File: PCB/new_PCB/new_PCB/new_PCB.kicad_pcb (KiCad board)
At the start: 2 copper layers, 127 x 102.2 mm, 18 parts, among them J1 XT60PW-F, J2 XT60PW-F, J3 MOLEX-Connector, J4 MOLEX-Connector, J5 MOLEX-Connector, J6 MOLEX-Connector, J7 MOLEX-Connector, J8 MOLEX-Connector, U1 ESP32-S3-DEVKITC-1-N16R8V

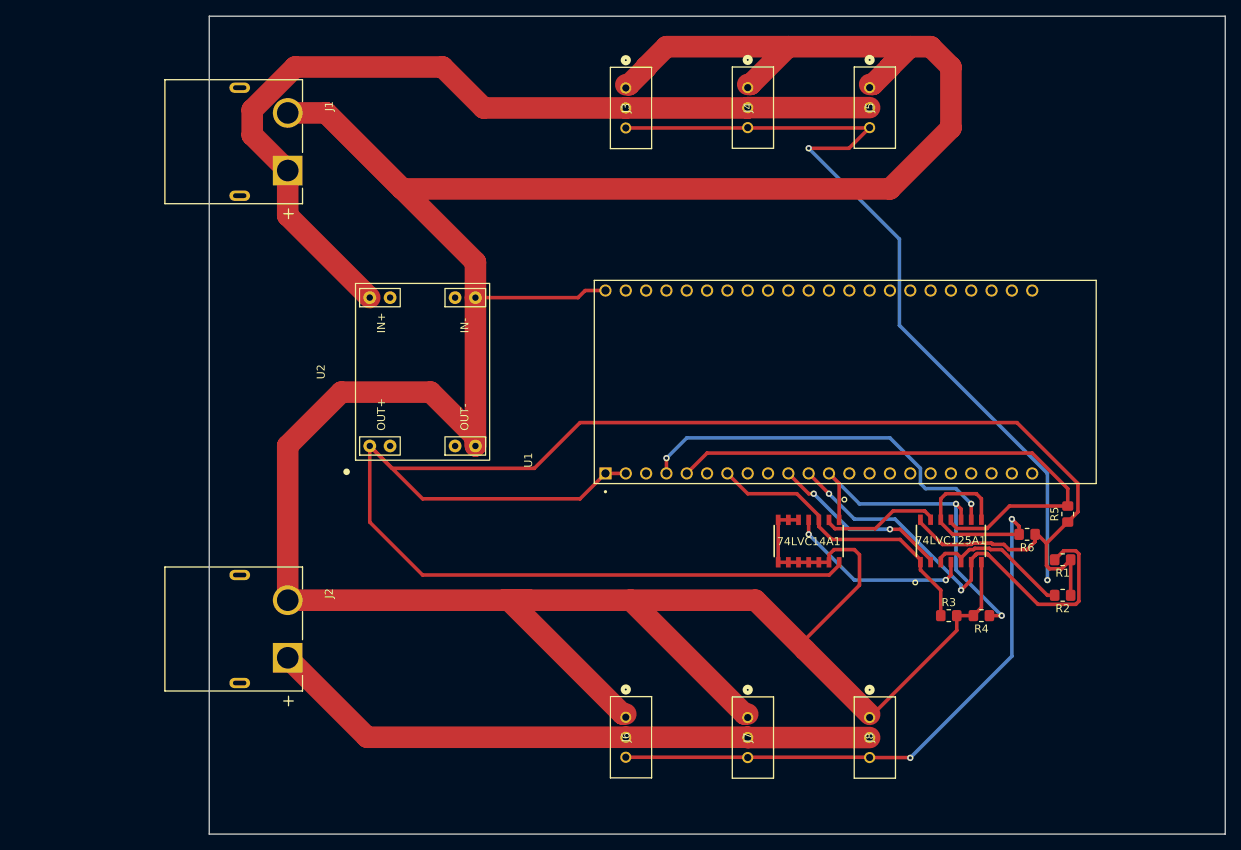
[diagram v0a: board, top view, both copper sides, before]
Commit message: Add changes to new pcb
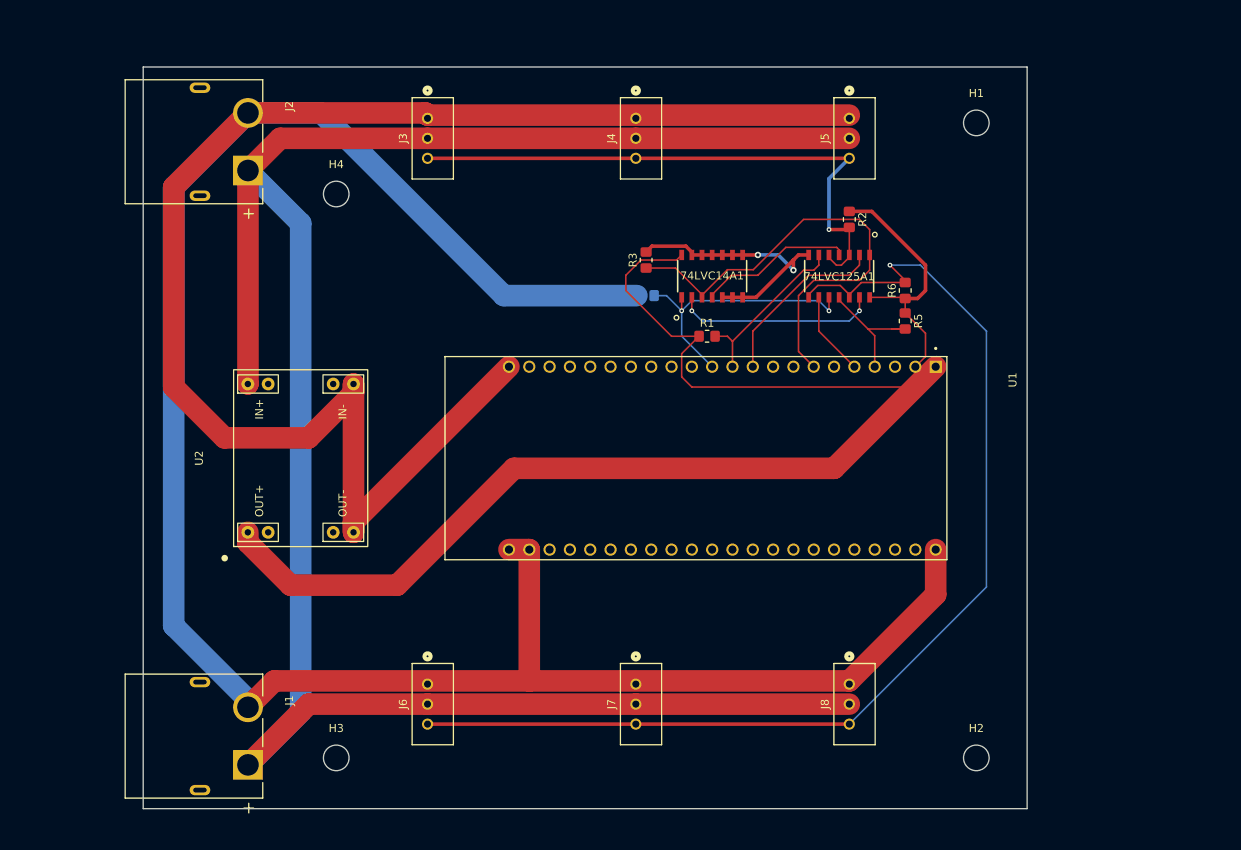
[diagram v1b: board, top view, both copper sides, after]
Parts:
- added H1: MountingHole, MountingHole:MountingHole_3.2mm_M3_ISO14580, F.Cu at (137.8, 29.8)
- added H2: MountingHole, MountingHole:MountingHole_3.2mm_M3_ISO14580, F.Cu at (137.8, 109.2)
- added H3: MountingHole, MountingHole:MountingHole_3.2mm_M3_ISO14580, F.Cu at (57.8, 109.2)
- added H4: MountingHole, MountingHole:MountingHole_3.2mm_M3_ISO14580, F.Cu at (57.8, 38.7)
- R4: moved to B.Cu
- moved J1 74.5 mm to (46.8, 106.5)
- moved J2 61.1 mm to (46.8, 32.2)
- moved R3 58.4 mm to (96.5, 47.0), turned to 90 degrees
- moved R4 57.9 mm to (96.5, 51.4)
- moved R2 54.0 mm to (121.9, 41.9), turned to -90 degrees
- moved R1 52.5 mm to (104.1, 56.5), turned to 0 degrees
- moved 74LVC125A1 38.9 mm to (124.5, 46.4), turned to -90 degrees
- moved R6 34.1 mm to (128.9, 50.8), turned to 90 degrees
- moved 74LVC14A1 34.1 mm to (101.0, 51.7), turned to 90 degrees
- moved R5 31.5 mm to (128.9, 54.6), turned to -90 degrees
- moved J6 25.1 mm to (69.2, 100.0)
- moved J3 25.1 mm to (69.2, 29.3)
- moved U1 21.0 mm to (102.7, 71.8), turned to -90 degrees
- moved U2 18.7 mm to (53.3, 71.8)
- moved J7 14.6 mm to (95.2, 100.0)
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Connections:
- U1 pad J1_22: (no net) -> GND
- U1 pad J1_4: /TX2 -> /RX2
- U1 pad J1_5: /RX2 -> /TX2
- U1 pad J3_21: (no net) -> GND
- U1 pad J3_22: (no net) -> GND
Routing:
- net VBUS: track 188.0 -> 261.6 mm
- net /RX2: track 69.1 -> 16.8 mm
- net /SERVO_DATA1: track 124.2 -> 72.7 mm, vias 2 -> 1
- net /SERVO_DATA2: track 94.6 -> 141.7 mm, vias 2 -> 1
- net +3.3V: track 242.5 -> 195.7 mm
- net /TX2: track 47.6 -> 10.5 mm, vias 2 -> 0
- net /RX1: track 56.1 -> 21.6 mm, vias 2 -> 0
- net GND: track 454.5 -> 480.1 mm, vias 0 -> 2
- net /TXEN1: track 37.4 -> 59.4 mm
- net /RXEN2: track 14.9 -> 25.4 mm, vias 0 -> 2
- net /TXEN2: track 43.9 -> 35.6 mm
- net /RXEN1: track 23.8 -> 19.4 mm, vias 2 -> 0
- net /TX1: vias 2 -> 0
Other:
- board size 127 x 102.2 mm -> 110.5 x 92.7 mm

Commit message: Final PCB version
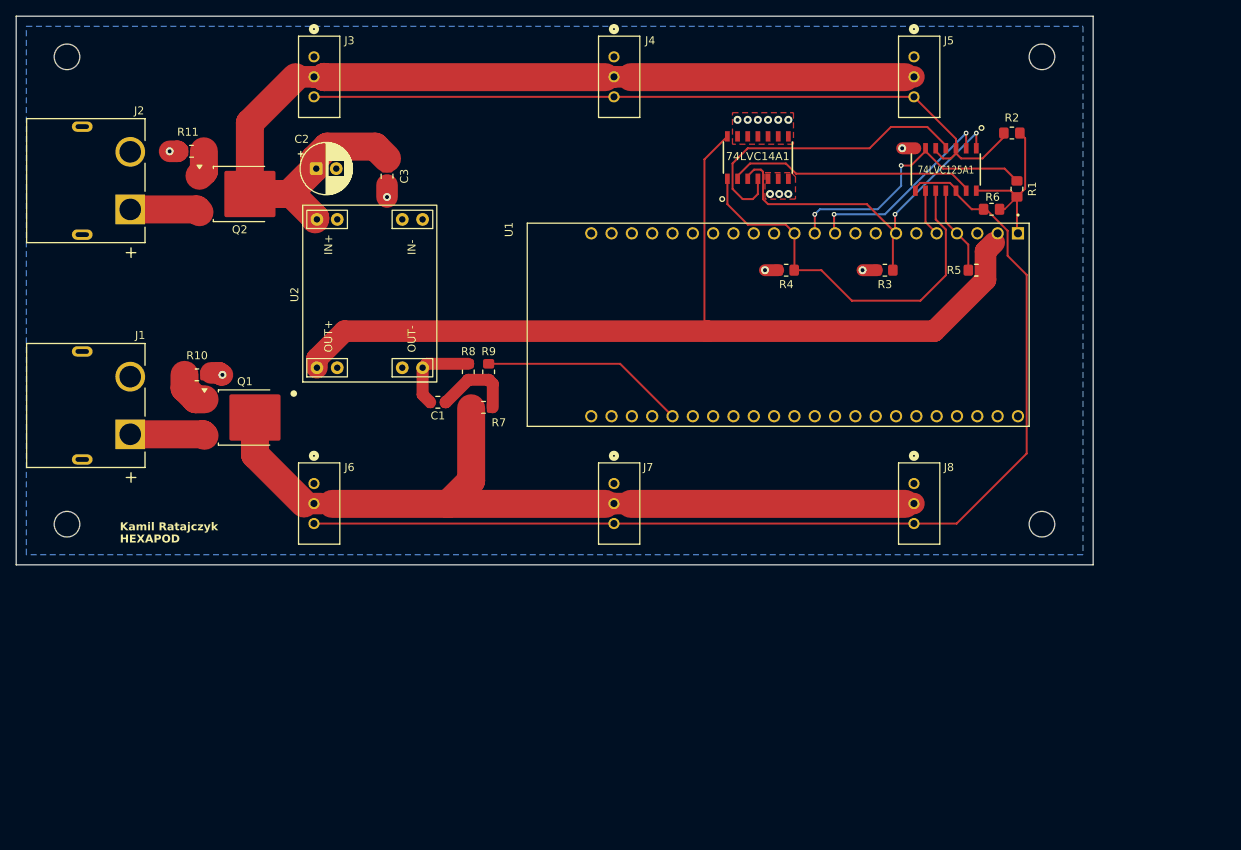
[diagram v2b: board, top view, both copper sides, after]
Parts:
- added C1: 100nF, Capacitor_SMD:C_0805_2012Metric, F.Cu at (70.5, 64.8)
- added C2: 100uF, Capacitor_THT:CP_Radial_D6.3mm_P2.50mm, F.Cu at (55.3, 35.6)
- added C3: 100nF, Capacitor_SMD:C_0805_2012Metric, F.Cu at (64.1, 36.5)
- added Q1: Q_PMOS, Package_TO_SOT_SMD:TO-252-2, F.Cu at (46.4, 66.7)
- added Q2: Q_PMOS, Package_TO_SOT_SMD:TO-252-2, F.Cu at (45.7, 38.7)
- added R10: 10k, Resistor_SMD:R_0805_2012Metric_Pad1.20x1.40mm_HandSolder, F.Cu at (40.4, 61.3)
- added R11: 10k, Resistor_SMD:R_0805_2012Metric_Pad1.20x1.40mm_HandSolder, F.Cu at (39.7, 33.4)
- added R7: 100k, Resistor_SMD:R_0805_2012Metric_Pad1.20x1.40mm_HandSolder, F.Cu at (76.2, 65.4)
- added R8: 22k, Resistor_SMD:R_0805_2012Metric_Pad1.20x1.40mm_HandSolder, F.Cu at (74.3, 61.0)
- added R9: 1k, Resistor_SMD:R_0805_2012Metric_Pad1.20x1.40mm_HandSolder, F.Cu at (76.8, 61.0)
- R4: moved to F.Cu
- moved H2 143.5 mm to (24.1, 21.6)
- moved H3 92.9 mm to (146.0, 80.0)
- moved H4 53.3 mm to (24.1, 80.0)
- moved J1 43.9 mm to (32.0, 65.2)
- moved R1 42.9 mm to (142.9, 38.1), turned to 90 degrees
- moved R3 29.9 mm to (126.4, 48.3), turned to 180 degrees
- moved J6 28.8 mm to (55.0, 74.9)
- moved J8 26.3 mm to (130.0, 74.9)
- moved J7 25.2 mm to (92.5, 74.9)
- moved R2 23.0 mm to (142.2, 31.1), turned to 180 degrees
- moved U2 22.3 mm to (62.0, 51.2)
- moved U1 19.6 mm to (113.0, 55.1)
- moved 74LVC125A1 18.9 mm to (137.8, 33.0)
- moved R4 17.8 mm to (114.0, 48.3)
- moved J3 16.1 mm to (55.0, 21.6)
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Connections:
- J1 pad 1: VBUS -> VBAT
- J2 pad 1: VBUS -> VBAT
- J3 pad 2: VBUS -> VBUS_2
- J4 pad 2: VBUS -> VBUS_2
- J5 pad 2: VBUS -> VBUS_2
- J6 pad 2: VBUS -> VBUS_1
- J7 pad 2: VBUS -> VBUS_1
- J8 pad 2: VBUS -> VBUS_1
- U1 pad J3_18: unconnected-(U1-GPIO21-PadJ3_18) -> /BAT_LVL
- U2 pad 8: VBUS -> VBUS_2
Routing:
- net GND: track 480.1 -> 19.8 mm, vias 2 -> 15
- net VBUS: track 261.6 -> 0.00 mm
- net VBUS_2: track 0.00 -> 119.6 mm
- net VBUS_1: track 0.00 -> 100.1 mm
- net +3.3V: track 195.7 -> 146.5 mm
- net /BAT_LVL: track 0.00 -> 25.7 mm
- net /SERVO_DATA1: track 72.7 -> 95.6 mm, vias 1 -> 0
- net /RXEN1: track 19.4 -> 38.9 mm
- net VBAT: track 0.00 -> 18.2 mm
- net /TXEN2: track 35.6 -> 50.6 mm, vias 2 -> 0
- net /RX1: track 21.6 -> 34.3 mm, vias 0 -> 2
- net /TXEN1: track 59.4 -> 48.0 mm, vias 0 -> 2
- net Net-(C1-Pad1): track 0.00 -> 10.2 mm
- net /RXEN2: track 25.4 -> 31.2 mm, vias 2 -> 0
- net /RX2: track 16.8 -> 11.1 mm
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- added copper zone on B.Cu, net GND
- added copper zone on F.Cu, net GND
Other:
- board size 110.5 x 92.7 mm -> 134.6 x 68.6 mm
- board text added: "HEXAPOD"
- board text added: "Kamil Ratajczyk"

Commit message: Final version of 2.0 PCB version
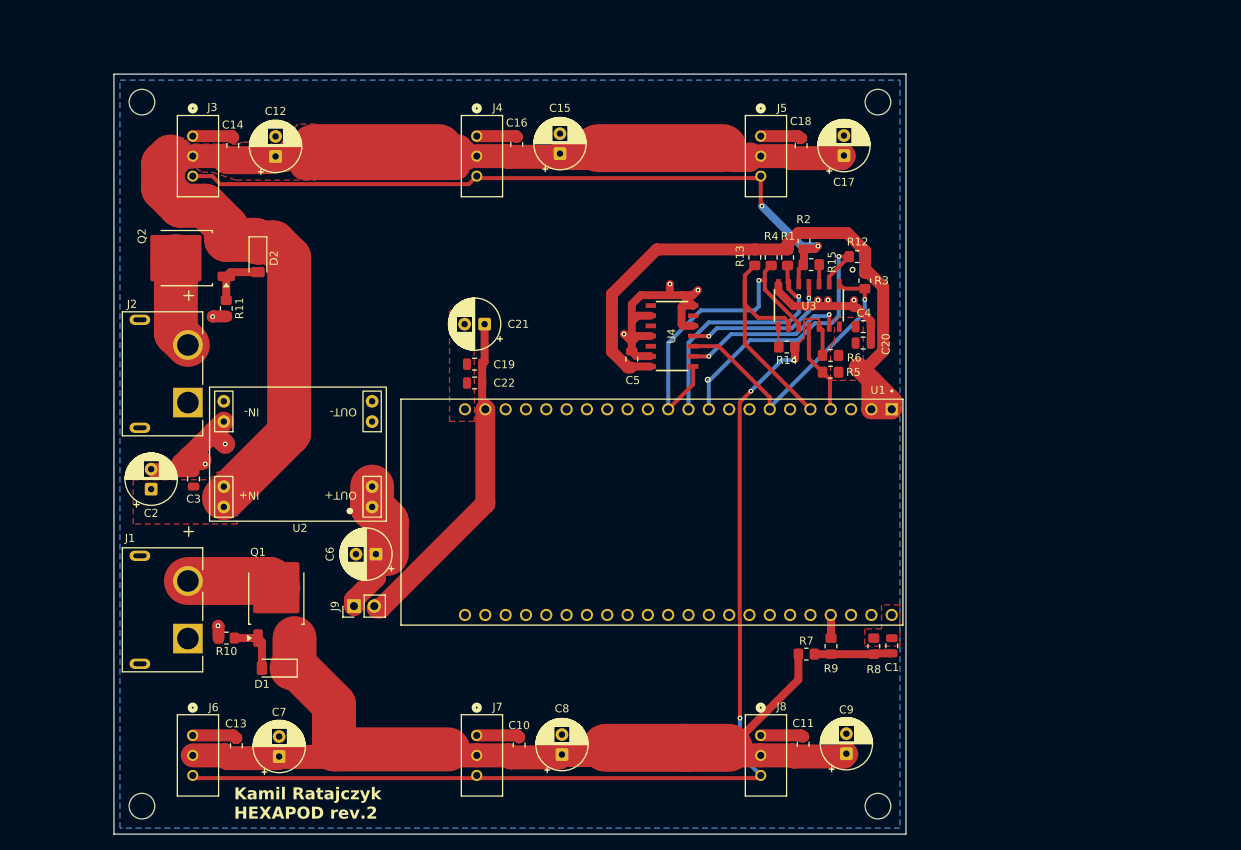
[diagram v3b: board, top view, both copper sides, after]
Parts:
- removed 74LVC125A1, 74LVC14A1: ~, Elements:SOT108-1
- added C10: 100nF, Capacitor_SMD:C_0805_2012Metric, F.Cu at (80.6, 107.6)
- added C11: 100nF, Capacitor_SMD:C_0805_2012Metric, F.Cu at (116.2, 107.5)
- added C12: 220uF, Capacitor_THT:CP_Radial_D6.3mm_P2.50mm, F.Cu at (50.2, 34.0)
- added C13: 100nF, Capacitor_SMD:C_0805_2012Metric, F.Cu at (45.3, 107.7)
- added C14: 100nF, Capacitor_SMD:C_0805_2012Metric, F.Cu at (44.9, 32.7)
- added C15: 220uF, Capacitor_THT:CP_Radial_D6.3mm_P2.50mm, F.Cu at (85.8, 33.7)
- added C16: 100nF, Capacitor_SMD:C_0805_2012Metric, F.Cu at (80.4, 32.5)
- added C17: 220uF, Capacitor_THT:CP_Radial_D6.3mm_P2.50mm, F.Cu at (121.2, 33.9)
- added C18: 100nF, Capacitor_SMD:C_0805_2012Metric, F.Cu at (115.9, 32.7)
- added C19: 10uF, Capacitor_SMD:C_0805_2012Metric, F.Cu at (75.1, 60.0)
- added C20: 10uF, Capacitor_SMD:C_0805_2012Metric, F.Cu at (123.7, 57.4)
- added C21: 220uF, Capacitor_THT:CP_Radial_D6.3mm_P2.50mm, F.Cu at (76.3, 55.0)
- added C22: 100nF, Capacitor_SMD:C_0805_2012Metric, F.Cu at (75.1, 62.4)
- added C4: 100nF, Capacitor_SMD:C_0805_2012Metric, F.Cu at (123.7, 55.3)
- added C5: 100nF, Capacitor_SMD:C_0805_2012Metric, F.Cu at (94.7, 59.4)
- added C6: 22uF, Capacitor_THT:CP_Radial_D6.3mm_P2.50mm, F.Cu at (62.8, 83.8)
- added C7: 220uF, Capacitor_THT:CP_Radial_D6.3mm_P2.50mm, F.Cu at (50.6, 109.0)
- added C8: 220uF, Capacitor_THT:CP_Radial_D6.3mm_P2.50mm, F.Cu at (86.0, 108.8)
- added C9: 220uF, Capacitor_THT:CP_Radial_D6.3mm_P2.50mm, F.Cu at (121.5, 108.7)
- added D1: BZV55B15, Diode_SMD:D_MiniMELF, F.Cu at (50.2, 98.0)
- added D2: BZV55B15, Diode_SMD:D_MiniMELF, F.Cu at (48.0, 46.8)
- added J9: Conn_01x02, Connector_PinHeader_2.54mm:PinHeader_1x02_P2.54mm_Vertical, F.Cu at (60.0, 90.2)
- added R12: 10k, Resistor_SMD:R_0805_2012Metric_Pad1.20x1.40mm_HandSolder, F.Cu at (122.9, 46.6)
- added R13: 10k, Resistor_SMD:R_0805_2012Metric_Pad1.20x1.40mm_HandSolder, F.Cu at (110.1, 46.7)
- added R14: 22R, Resistor_SMD:R_0805_2012Metric_Pad1.20x1.40mm_HandSolder, F.Cu at (114.1, 57.9)
- added R15: 22R, Resistor_SMD:R_0805_2012Metric_Pad1.20x1.40mm_HandSolder, F.Cu at (117.2, 47.6)
- added U3: 74LVC125A1, Elements:SOT108-1, F.Cu at (120.7, 50.0)
- added U4: 74LVC14A1, Elements:SOT108-1, F.Cu at (102.4, 60.3)
- Q1, Q2: value Q_PMOS -> SUD50P04-08
- moved H1 146.4 mm to (33.5, 115.2)
- moved H2 138.0 mm to (125.5, 115.2)
- moved C1 64.4 mm to (127.2, 95.2), turned to 90 degrees
- moved R8 61.2 mm to (125.0, 95.3)
- moved H3 56.6 mm to (125.5, 27.2)
- moved R9 54.8 mm to (119.6, 95.3)
- moved H4 53.6 mm to (33.5, 27.2)
- moved R7 50.8 mm to (116.5, 96.2)
- moved C2 45.1 mm to (34.6, 75.6), turned to 90 degrees
- moved C3 44.9 mm to (40.0, 74.3), turned to 90 degrees
- moved J8 36.8 mm to (110.8, 106.4)
- moved J7 35.8 mm to (75.3, 106.4)
- moved J6 34.9 mm to (39.8, 106.4)
- moved R10 33.1 mm to (44.1, 94.2), turned to 180 degrees
- moved R1 29.9 mm to (114.2, 46.7), turned to -90 degrees
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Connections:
- net Net-(C1-Pad1) renamed /BAT_LVL_DIV
- net Net-(Q1-G) renamed /Q1_GATE
- net Net-(Q2-G) renamed /Q2_GATE
- J1 pad 1: VBAT -> VBAT_1
- J2 pad 1: VBAT -> VBAT_2
- Q1 pad 2: VBUS_1 -> VBAT_1
- Q1 pad 3: VBAT -> VBUS_1
- Q2 pad 2: VBUS_2 -> VBAT_2
- Q2 pad 3: VBAT -> VBUS_2
- R1 pad 1: +3.3V -> +3V3
- R2 pad 1: +3.3V -> +3V3
- R3 pad 1: /TXEN1 -> +3V3
- R3 pad 2: GND -> /TXEN1
- R4 pad 1: /TXEN2 -> +3V3
- R4 pad 2: GND -> /TXEN2
- R5 pad 1: +3.3V -> +3V3
- R6 pad 1: +3.3V -> +3V3
- U1 pad J1_1: +3.3V -> +3V3
- U1 pad J1_2: +3.3V -> +3V3
- U1 pad J1_21: unconnected-(U1-5V0-PadJ1_21) -> +5V
- U1 pad J3_18: /BAT_LVL -> unconnected-(U1-GPIO21-PadJ3_18)
- U1 pad J3_4: unconnected-(U1-GPIO1-PadJ3_4) -> /BAT_LVL
- U2 pad 1: +3.3V -> /+5V_RAW
- U2 pad 2: unconnected-(U2-OUT+-Pad2) -> /+5V_RAW
- U2 pad 3: unconnected-(U2-OUT--Pad3) -> GND
- U2 pad 6: unconnected-(U2-IN--Pad6) -> GND
- U2 pad 7: unconnected-(U2-IN+-Pad7) -> VBUS_2
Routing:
- net +3.3V: track 146.5 -> 0.00 mm
- net GND: track 19.8 -> 109.6 mm, vias 15 -> 10
- net +3V3: track 0.00 -> 80.3 mm
- net +5V: track 0.00 -> 41.7 mm
- net VBUS_2: track 119.6 -> 158.9 mm
- net /TX2: track 5.91 -> 31.9 mm
- net /BAT_LVL: track 25.7 -> 2.91 mm
- net VBUS_1: track 100.1 -> 121.0 mm
- net /RXEN1: track 38.9 -> 19.1 mm, vias 0 -> 2
- net VBAT: track 18.2 -> 0.00 mm
- net /+5V_RAW: track 0.00 -> 16.8 mm
- net VBAT_2: track 0.00 -> 11.7 mm
- net VBAT_1: track 0.00 -> 11.6 mm
- net /TX1: track 25.1 -> 36.4 mm, vias 2 -> 1
- net /TXEN1: track 48.0 -> 37.1 mm, vias 2 -> 1
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- added copper zone on F.Cu, net +3V3
- added copper zone on F.Cu, net VBUS_2
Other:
- board size 134.6 x 68.6 mm -> 99 x 95 mm
- board text added: "Kamil Ratajczyk HEXAPOD rev.2"
- board text removed: "HEXAPOD"
- board text removed: "Kamil Ratajczyk"
